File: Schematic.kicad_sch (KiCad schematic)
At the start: 13 parts, among them M1 Motor_Servo, M2 Motor_DC, U1 ESP32-WROOM-32D, U2 TF-Mini, U3 DC-DC Buck, U4 L298N Module, U5 TF-Mini, U6 TF-Mini, U7 TF-Mini, U9 LM337

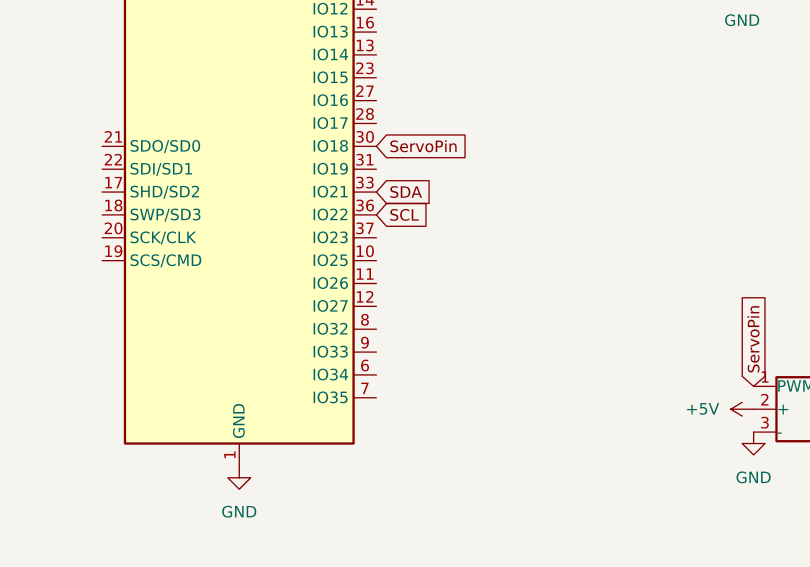
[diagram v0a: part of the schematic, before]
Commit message: continue docs
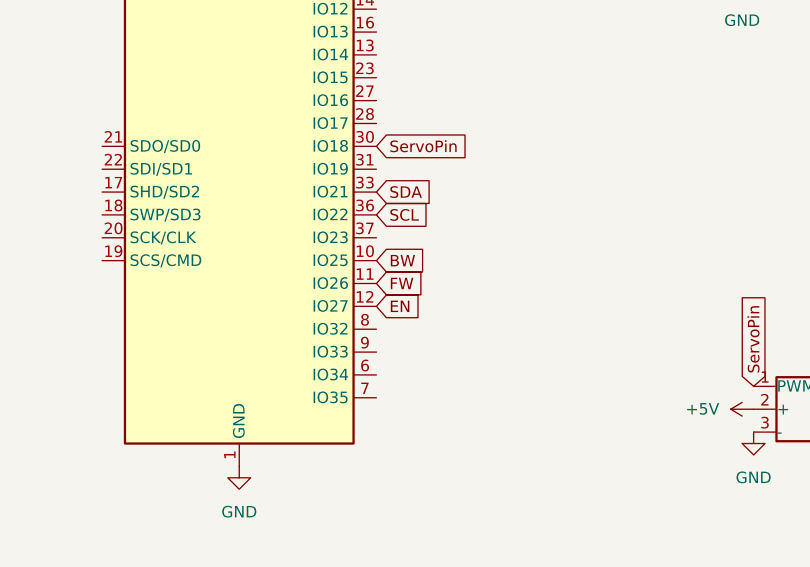
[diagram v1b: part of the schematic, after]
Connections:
- net BW: now also U1.10 (IO25)
- net EN: now also U1.12 (IO27)
- net FW: now also U1.11 (IO26)
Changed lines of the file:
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@@
+		)
+	)
+	(global_label "EN"
+		(shape input)
+		(at 69.85 87.63 0)
+		(fields_autoplaced yes)
+		(effects
+			(font
+				(size 1.27 1.27)
+			)
+			(justify left)
+		)
+		(property "Intersheetrefs" "${INTERSHEET_REFS}"
+			(at 75.3147 87.63 0)
+			(effects
+				(font
+					(size 1.27 1.27)
+				)
+				(justify left)
+				(hide yes)
+			)
 		)
 	)
@@
 				(hide yes)
 			)
+		)
+	)
+	(global_label "FW"
+		(shape input)
+		(at 69.85 85.09 0)
+		(fields_autoplaced yes)
+		(effects
+			(font
+				(size 1.27 1.27)
+			)
+			(justify left)
+		)
+		(property "Intersheetrefs" "${INTERSHEET_REFS}"
+			(at 75.3752 85.09 0)
+			(effects
+				(font
+					(size 1.27 1.27)
+				)
+				(justify left)
+				(hide yes)
+			)
+		)
+	)
+	(global_label "BW"
+		(shape input)
+		(at 69.85 82.55 0)
+		(fields_autoplaced yes)
+		(effects
+			(font
+				(size 1.27 1.27)
+			)
+			(justify left)
+		)
+		(property "Intersheetrefs" "${INTERSHEET_REFS}"
+			(at 75.5566 82.55 0)
+			(effects
+				(font
+					(size 1.27 1.27)
+				)
+				(justify left)
+				(hide yes)
+			)
